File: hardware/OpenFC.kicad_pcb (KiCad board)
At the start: 6 copper layers, 38.9 x 38.9 mm, 165 parts, among them J1 5V, J10 5V, J11 5V, J12 5V, J13 5V, J14 5V, J15 5V, J16 5V, J17 5V, J18 5V, J19 5V, J2 5V, J20 5V, J21 5V, J22 5V, J23 5V, J24 5V, J25 5V, J26 5V, J27 5V, J28 5V, J29 5V, J3 5V, J30 5V, J31 5V, J32 5V, J33 5V, J34 5V, J35 5V, J36 5V, J37 5V, J38 5V, J39 5V, J4 5V, J40 5V, J41 5V, J42 5V, J43 5V, J44 5V, J47 5V, J48 5V, J49 5V, J5 5V, J50 5V, J51 5V, J52 5V, J53 5V, J54 5V, J55 5V, J6 5V, J7 5V, J8 5V, J9 5V, P1 SM08B-SRSS-TB(LF)(SN), Q1 AP1606, Q2 AP1606, U1 TS2306A 240GF MSM 9_C2976675, U10 SN74LVC1G3157DTBR, U11 COS8051SOT, U12 TLV7031DPWR, U2 RP2354B_C39843328, U3 TI LMR51430YFDDCR, U4 TI LMR51430YFDDCR, U5 TPS2116DRLR, U6 NCV8187AMT180TAG, U7 LP5912-3.3DRVR, U8 SM06B-SRSS-TB(LF)(SN), U9 LSM6DSV16XTR, X1 XTM25012000JT00351001

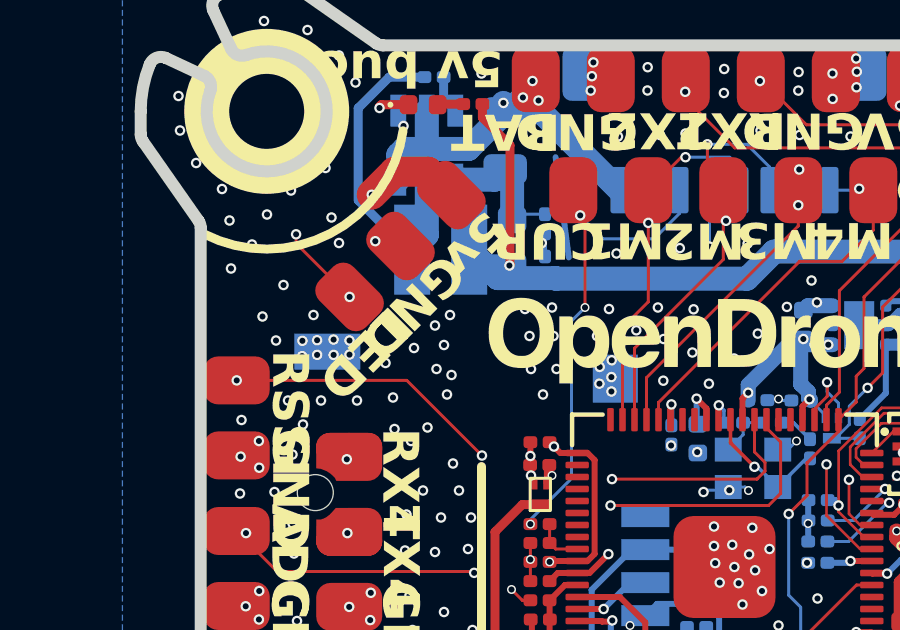
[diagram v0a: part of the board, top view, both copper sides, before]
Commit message: cleanup
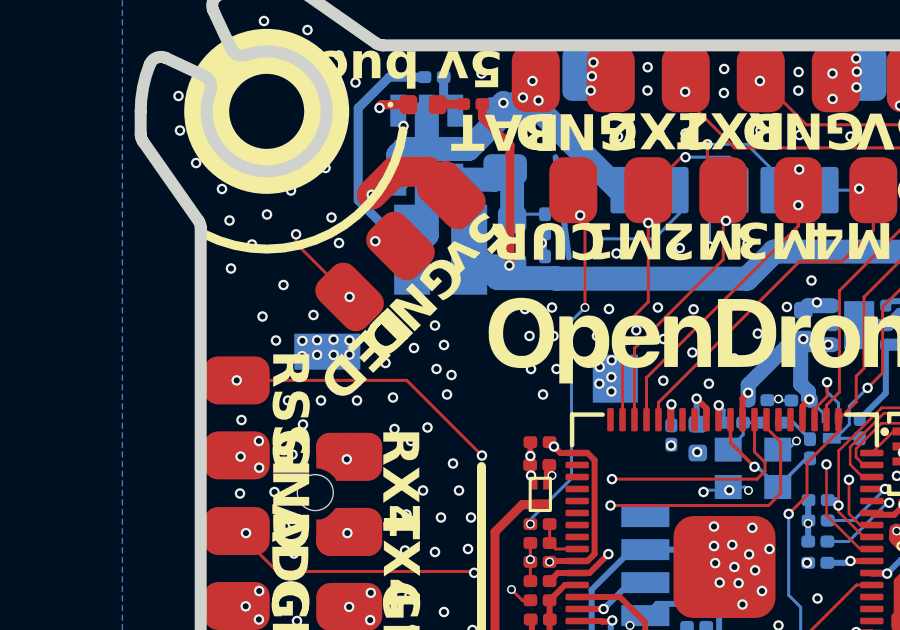
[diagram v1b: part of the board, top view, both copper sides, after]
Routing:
- net +3.3V: track 49.1 -> 61.0 mm, vias 23 -> 22
- added copper zone on In2.Cu, net GND
- removed copper zone on In2.Cu, net +3.3V
